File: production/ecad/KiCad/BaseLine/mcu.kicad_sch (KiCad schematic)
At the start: 45 parts, among them J2 1332645, Q1 AO3400A, Q2 AO3400A, SW1 SW_Push, SW2 SW_Push, U2 ESP32-WROOM-32UE_M113EH6400UH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, U3 CP2102N-A02-GQFN28

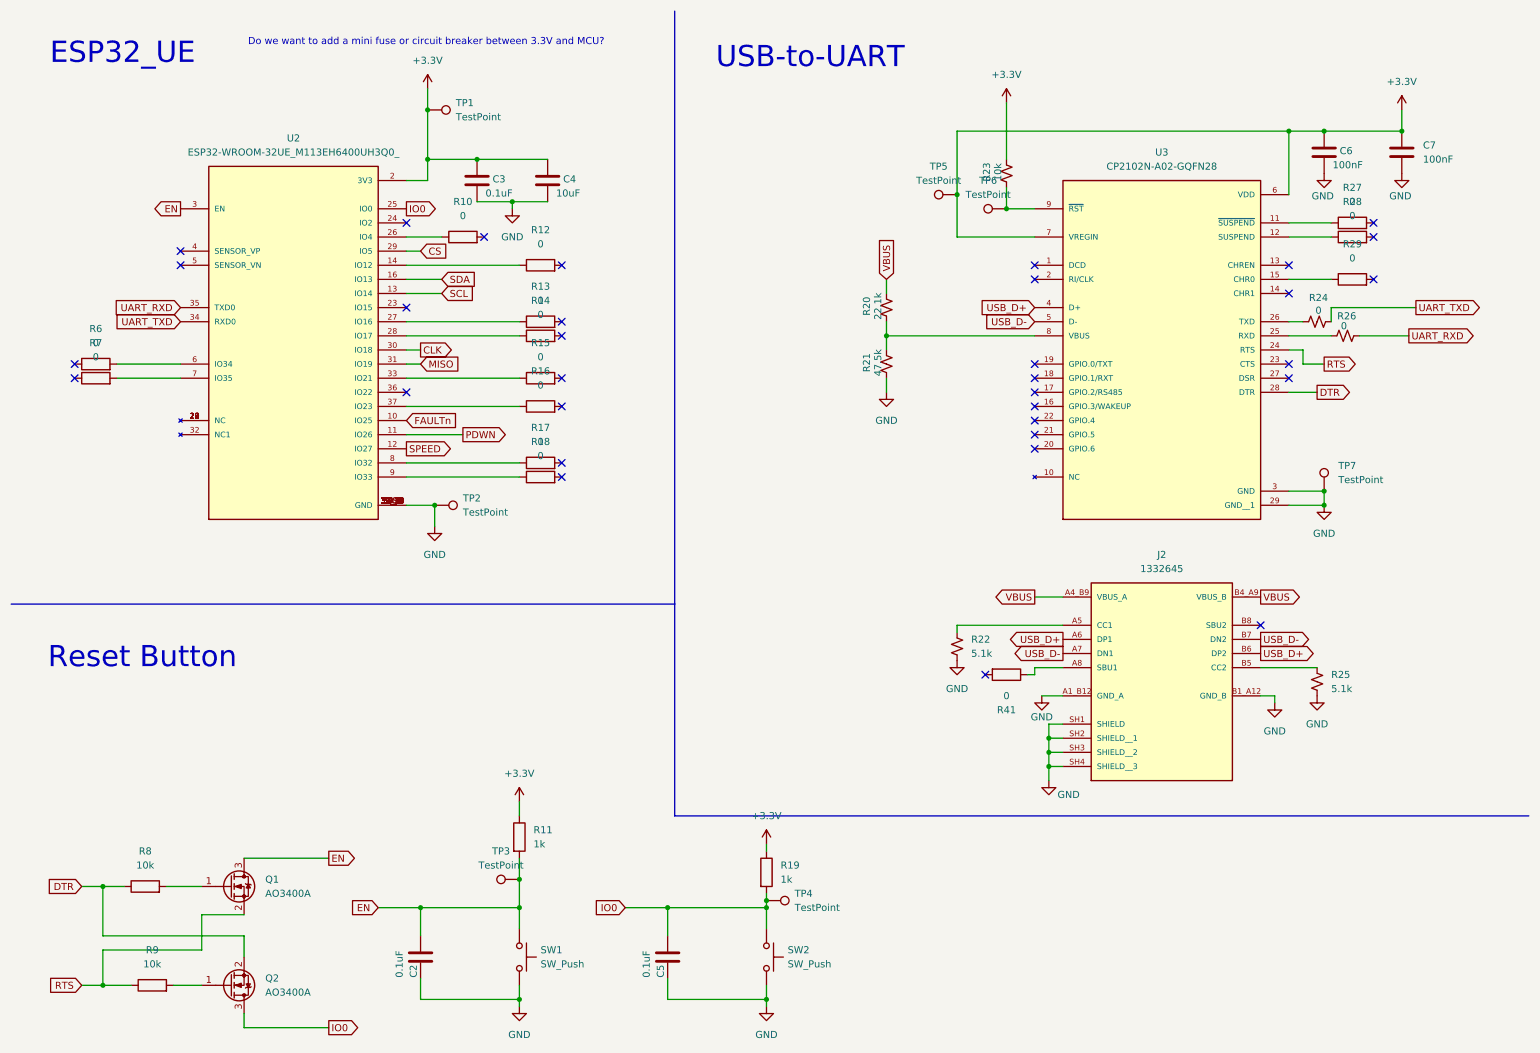
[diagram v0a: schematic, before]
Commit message: Rohi changes
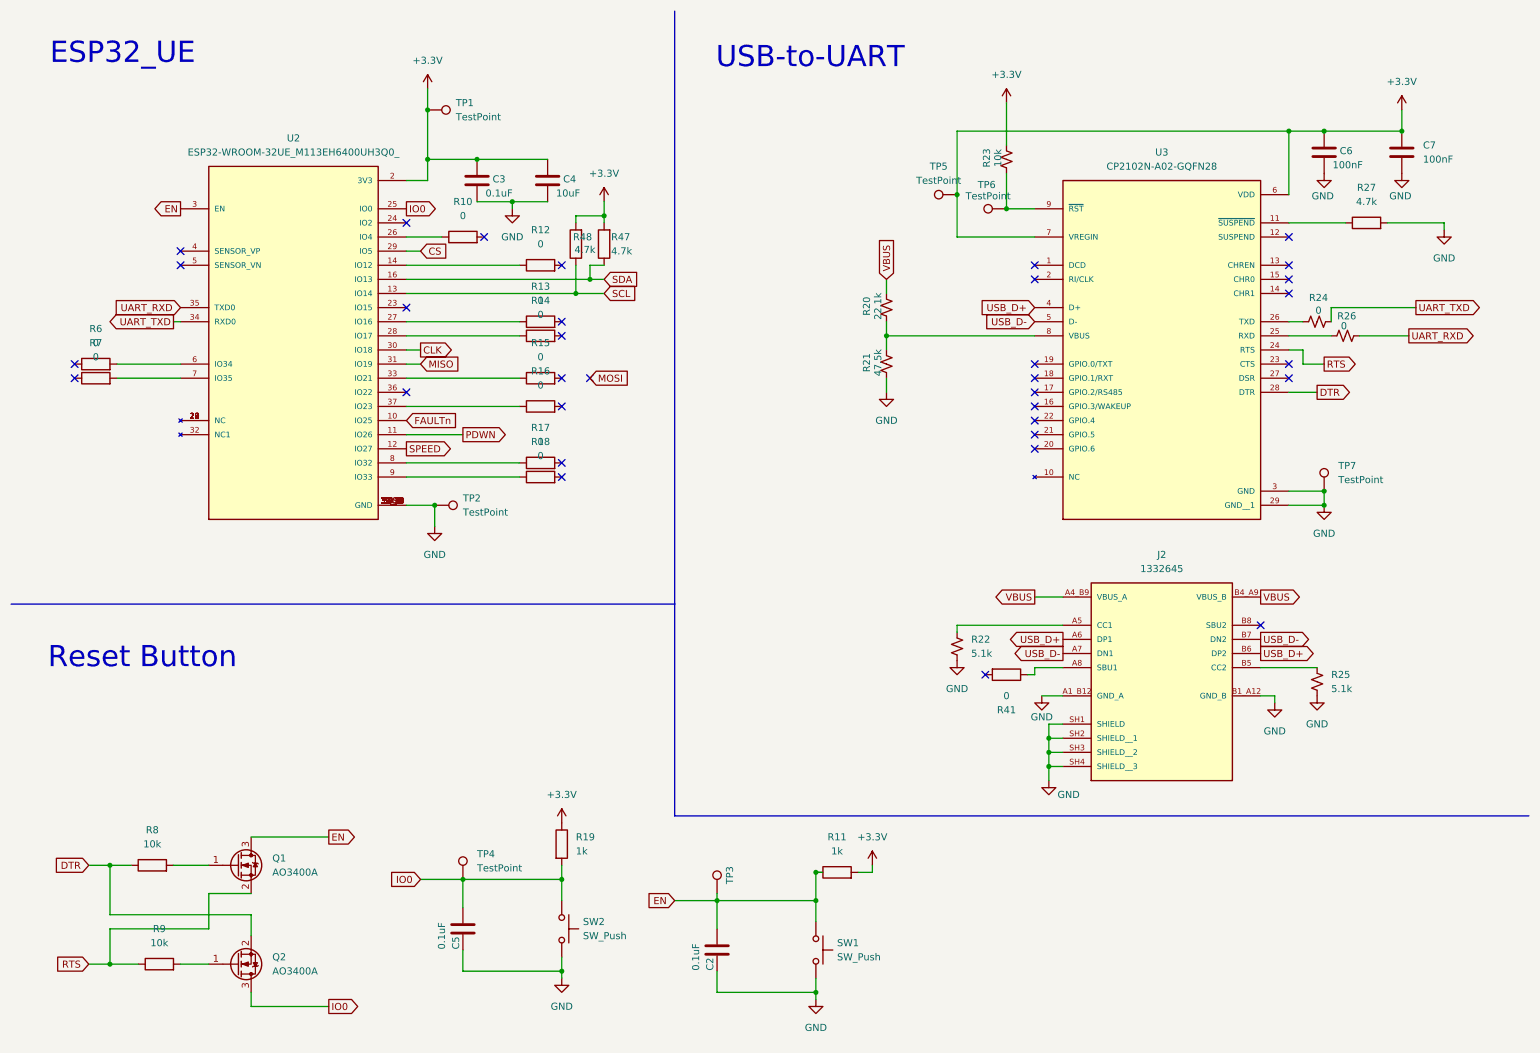
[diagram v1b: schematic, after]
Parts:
- removed R28, R29: 0, Resistor_SMD:R_0805_2012Metric, symbol Device:R
- added R47, R48: 4.7k, Resistor_SMD:R_0805_2012Metric, symbol Device:R
- R27: value 0 -> 4.7k
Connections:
- net +3.3V: now also R11.2, R47.2, R48.2; no longer R11.1
- net EN: now also R11.1; no longer R11.2
- net GND: now also R27.2
- net SCL: now also R48.1
- net SDA: now also R47.1
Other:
- note removed: "Do we want to add a mini fuse or circuit breaker between 3.3V and MCU?"
- moved on the sheet: C2, C5, Q1, Q2, R11, R19, R23, R27, R8, R9, SW1, SW2
